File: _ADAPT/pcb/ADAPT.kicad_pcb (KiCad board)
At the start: 4 copper layers, 68.6 x 53.3 mm, 17 parts, among them J1 VBAT, J2 VBAT, J3 VBAT, J4 Conn_01x02, J5 Conn_01x02

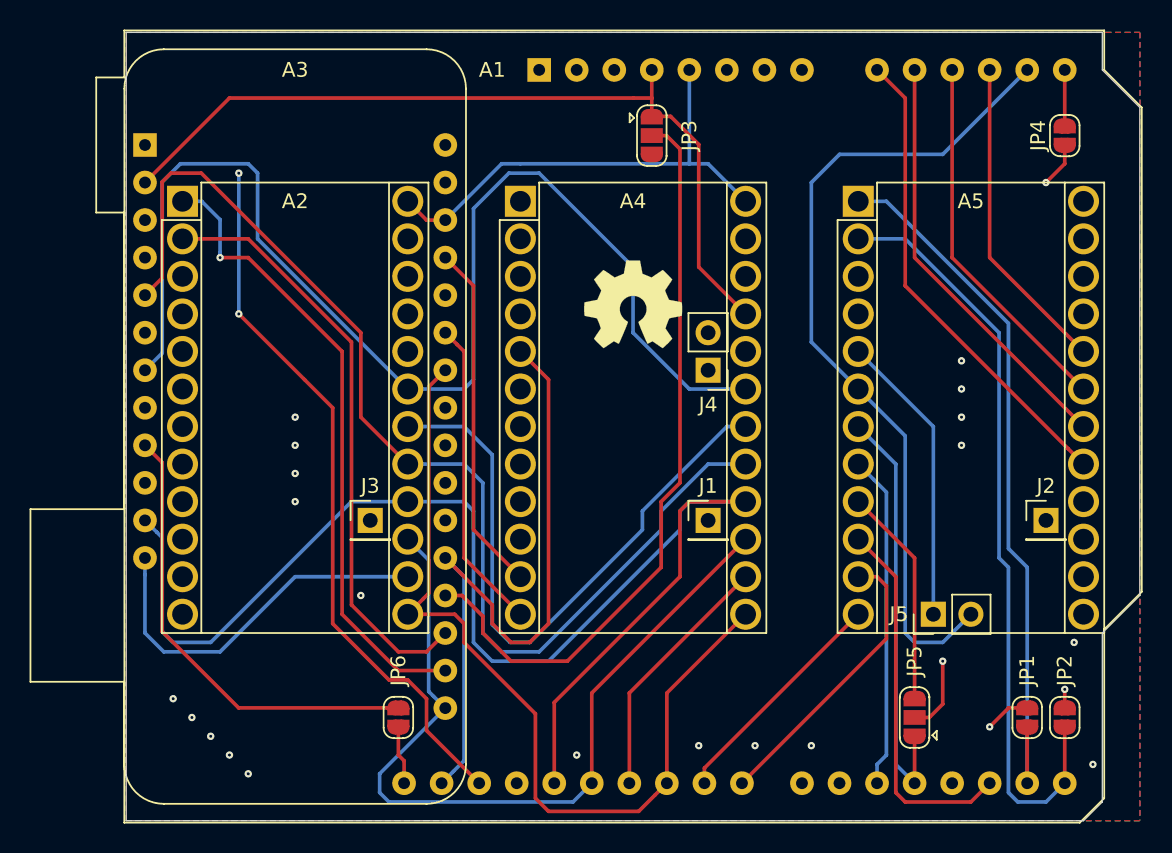
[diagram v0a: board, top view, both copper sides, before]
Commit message: cleanup using licenses
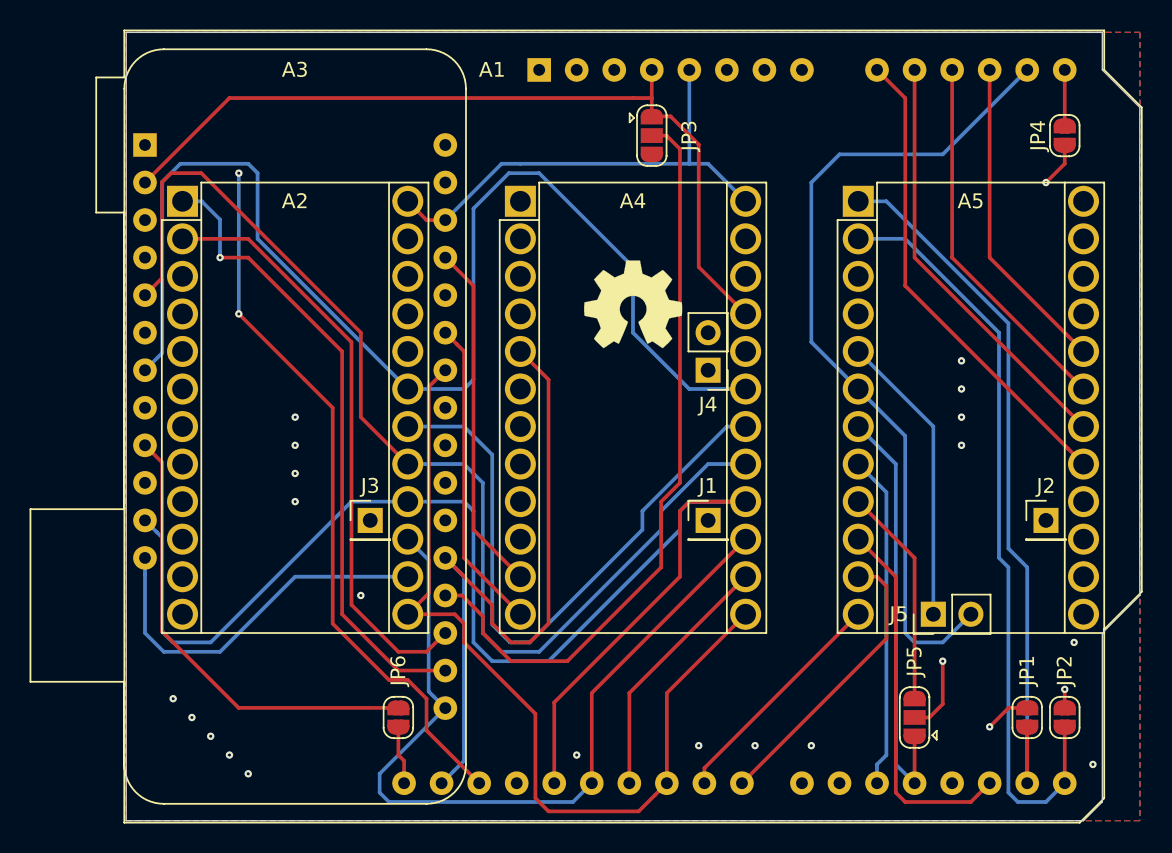
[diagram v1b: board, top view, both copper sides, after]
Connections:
- net ~RST renamed ~{RST}
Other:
- net class Default removed
- net class Power removed
- net class small removed
- net class tiny removed
